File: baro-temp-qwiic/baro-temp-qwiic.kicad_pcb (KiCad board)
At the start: 2 copper layers, 9 x 15 mm, 8 parts, among them J1 Conn_01x04_Male, U1 BMP388, U2 TMP102xxDRL

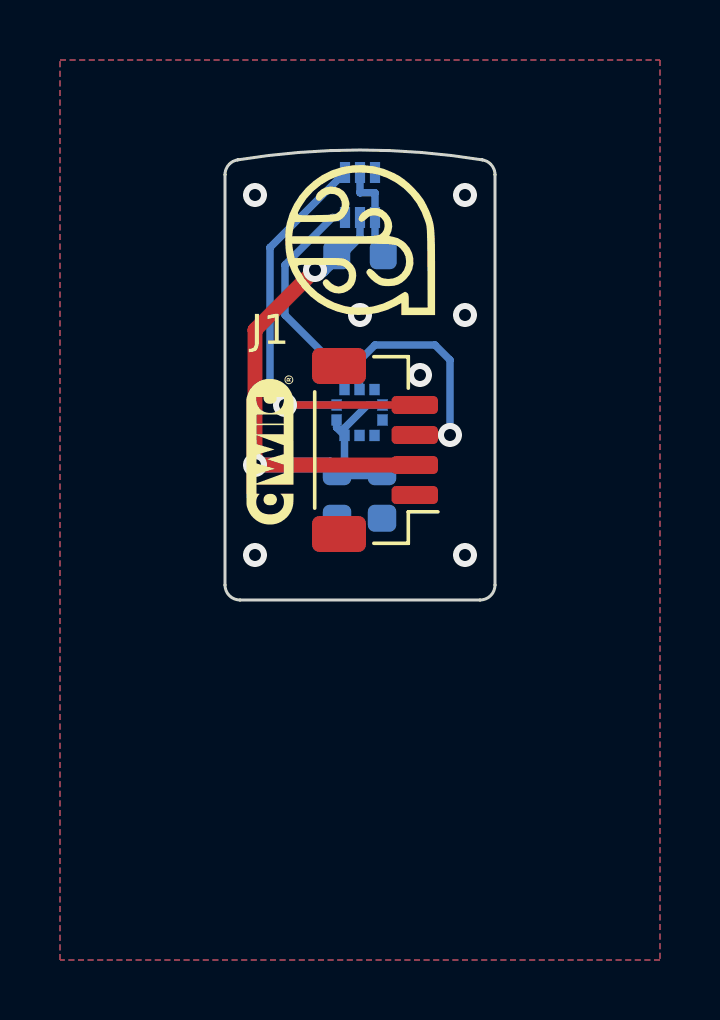
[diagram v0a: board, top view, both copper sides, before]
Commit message: Finished design and made fab outputs.
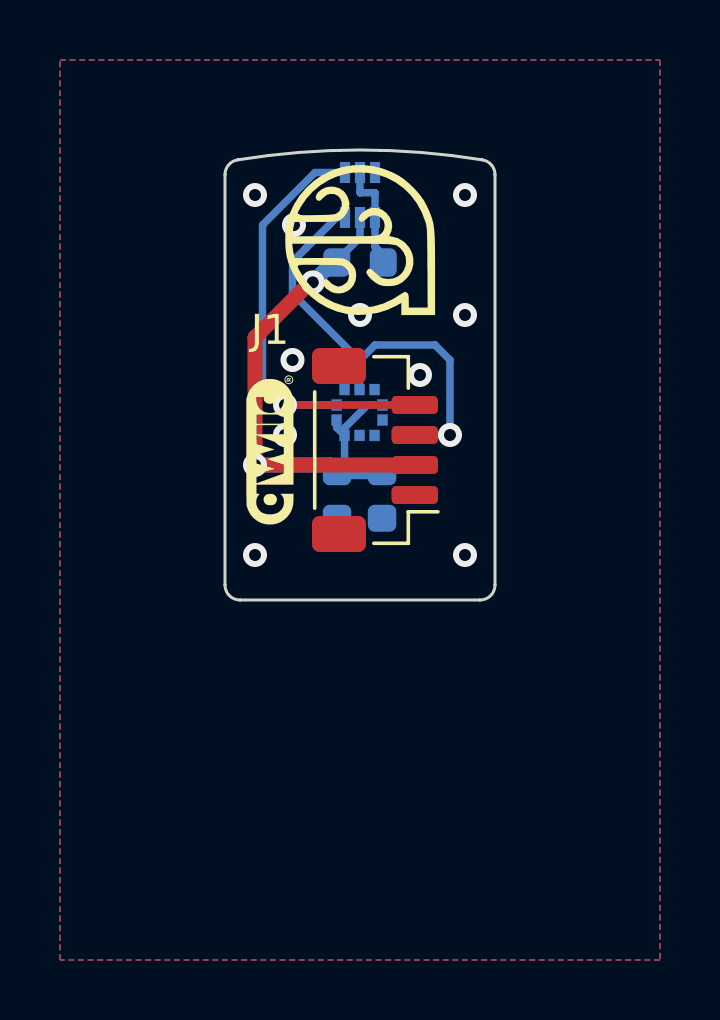
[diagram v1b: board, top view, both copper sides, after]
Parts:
- moved C3 0.25 mm to (0.00, -18.2)
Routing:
- net /SDA: track 15.5 -> 14.7 mm
- net /SCL: track 15.0 -> 15.8 mm
- net GND: vias 7 -> 10
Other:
- board text added: "Airball Temp/Baro 2023-03-14"
- board text added: "Copyright © 2023, The Airball authors"
- board text removed: "Airball Temp/Baro 2023-03-04"
- board text removed: "Copyright (C) 2023, The Airball Authors"
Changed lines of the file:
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@@
       (outputformat 1)
       (mirror false)
-      (drillshape 1)
+      (drillshape 0)
       (scaleselection 1)
       (outputdirectory "")
@@
     (pad "4" smd roundrect (at 1.5 1.325 90) (size 0.6 1.55) (layers "F.Cu" "F.Paste" "F.Mask") (roundrect_rratio 0.25)
       (net 4 "/SCL") (pinfunction "Pin_4") (pintype "passive"))
-    (pad "MP" smd roundrect (at 2.8 -1.2 90) (size 1.2 1.8) (layers "F.Cu" "F.Paste" "F.Mask") (roundrect_rratio 0.208333))
-    (pad "MP" smd roundrect (at -2.8 -1.2 90) (size 1.2 1.8) (layers "F.Cu" "F.Paste" "F.Mask") (roundrect_rratio 0.208333))
+    (pad "MP" smd roundrect (at 2.8 -1.2 90) (size 1.2 1.8) (layers "F.Cu" "F.Paste" "F.Mask") (roundrect_rratio 0.2083333333))
+    (pad "MP" smd roundrect (at -2.8 -1.2 90) (size 1.2 1.8) (layers "F.Cu" "F.Paste" "F.Mask") (roundrect_rratio 0.2083333333))
     (model "/home/ihab/airball-hardware/lib/airball-hardware.pretty/BM04B-SRSS.step"
       (offset (xyz 0 1.25 0))
@@
   )
   (footprint "Capacitor_SMD:C_0603_1608Metric" (layer "B.Cu")
-    (at 0 -18.5)
+    (at 0 -18.25)
     (descr "Capacitor SMD 0603 (1608 Metric), square (rectangular) end terminal, IPC_7351 nominal, (Body size source: IPC-SM-782 page 76, https://www.pcb-3d.com/wordpress/wp-content/uploads/ipc-sm-782a_amendment_1_and_2.pdf), generated with kicad-footprint-generator")
     (tags "capacitor")
@@
   (gr_line (start 4.5 -7.5) (end 4.5 -21.176615) (layer "Edge.Cuts") (width 0.1))
   (gr_arc (start 4.080321 -21.670121) (mid 4.380896 -21.500528) (end 4.5 -21.176615) (layer "Edge.Cuts") (width 0.1))
-  (gr_text "Airball Temp/Baro\n2023-03-04" (at -3 -14.5 90) (layer "B.SilkS")
+  (gr_text "Airball Temp/Baro\n2023-03-14" (at -3 -14.5 90) (layer "B.SilkS")
     (effects (font (size 0.5 0.5) (thickness 0.0625)) (justify mirror))
   )
-  (gr_text "Copyright (C) 2023,\nThe Airball Authors" (at 3 -15 90) (layer "B.SilkS")
+  (gr_text "Copyright © 2023,\nThe Airball authors" (at 3 -15 90) (layer "B.SilkS")
     (effects (font (size 0.5 0.5) (thickness 0.0625)) (justify mirror))
   )
-  (segment (start -3.5 -11.5) (end -3.5 -16) (width 0.5) (layer "F.Cu") (net 1))
-  (segment (start -3.5 -16) (end -1.5 -18) (width 0.5) (layer "F.Cu") (net 1))
+  (segment (start -1.663248 -17.586752) (end -3.5 -15.75) (width 0.5) (layer "F.Cu") (net 1))
+  (segment (start -1.5755 -17.586752) (end -1.663248 -17.586752) (width 0.5) (layer "F.Cu") (net 1))
+  (segment (start -3.5 -15.75) (end -3.5 -11.5) (width 0.5) (layer "F.Cu") (net 1))
   (segment (start 1.825 -11.5) (end -3.5 -11.5) (width 0.5) (layer "F.Cu") (net 1))
   (via (at -3.5 -11.5) (size 0.8) (drill 0.4) (layers "F.Cu" "B.Cu") (net 1))
-  (via (at -1.5 -18) (size 0.8) (drill 0.4) (layers "F.Cu" "B.Cu") (net 1))
+  (via (at -1.5755 -17.586752) (size 0.8) (drill 0.4) (layers "F.Cu" "B.Cu") (net 1))
+  (segment (start -1.5755 -17.586752) (end -0.912252 -18.25) (width 0.5) (layer "B.Cu") (net 1))
   (segment (start -0.780192 -13) (end -0.780192 -12.75) (width 0.25) (layer "B.Cu") (net 1))
   (segment (start -0.765192 -11.275) (end 0.734808 -11.275) (width 0.5) (layer "B.Cu") (net 1))
   (segment (start 0 -19.75) (end 0 -19.08) (width 0.25) (layer "B.Cu") (net 1))
-  (segment (start -1.5 -18) (end -1.275 -18) (width 0.5) (layer "B.Cu") (net 1))
   (segment (start -0.780192 -12.75) (end -0.515192 -12.485) (width 0.25) (layer "B.Cu") (net 1))
   (segment (start 0.25 -13.5) (end 0.749808 -13.5) (width 0.25) (layer "B.Cu") (net 1))
-  (segment (start -1.275 -18) (end -0.775 -18.5) (width 0.5) (layer "B.Cu") (net 1))
-  (segment (start -0.58 -18.5) (end -0.775 -18.5) (width 0.25) (layer "B.Cu") (net 1))
   (segment (start 0 -19.08) (end -0.58 -18.5) (width 0.25) (layer "B.Cu") (net 1))
   (segment (start -0.990192 -11.5) (end -0.765192 -11.275) (width 0.5) (layer "B.Cu") (net 1))
   (segment (start -0.515192 -11.525) (end -0.765192 -11.275) (width 0.25) (layer "B.Cu") (net 1))
+  (segment (start -0.912252 -18.25) (end -0.775 -18.25) (width 0.5) (layer "B.Cu") (net 1))
   (segment (start -0.515192 -12.485) (end -0.515192 -11.525) (width 0.25) (layer "B.Cu") (net 1))
   (segment (start -0.515192 -12.485) (end -0.515192 -12.734808) (width 0.25) (layer "B.Cu") (net 1))
@@
   (segment (start -0.515192 -12.734808) (end 0.25 -13.5) (width 0.25) (layer "B.Cu") (net 1))
   (via (at -3.5 -20.5) (size 0.8) (drill 0.4) (layers "F.Cu" "B.Cu") (free) (net 2))
+  (via (at -2.25 -15) (size 0.8) (drill 0.4) (layers "F.Cu" "B.Cu") (free) (net 2))
   (via (at -3.5 -8.5) (size 0.8) (drill 0.4) (layers "F.Cu" "B.Cu") (free) (net 2))
   (via (at 3.5 -16.5) (size 0.8) (drill 0.4) (layers "F.Cu" "B.Cu") (free) (net 2))
+  (via (at -2.5 -12.5) (size 0.8) (drill 0.4) (layers "F.Cu" "B.Cu") (free) (net 2))
   (via (at 3.5 -8.5) (size 0.8) (drill 0.4) (layers "F.Cu" "B.Cu") (free) (net 2))
   (via (at 2 -14.5) (size 0.8) (drill 0.4) (layers "F.Cu" "B.Cu") (free) (net 2))
   (via (at 3.5 -20.5) (size 0.8) (drill 0.4) (layers "F.Cu" "B.Cu") (free) (net 2))
   (via (at 0 -16.5) (size 0.8) (drill 0.4) (layers "F.Cu" "B.Cu") (free) (net 2))
+  (via (at -2.2 -19.5) (size 0.8) (drill 0.4) (layers "F.Cu" "B.Cu") (free) (net 2))
   (segment (start 0 -21.25) (end 0 -20.58) (width 0.25) (layer "B.Cu") (net 2))
   (segment (start 0.5 -19.75) (end 0.5 -18.775) (width 0.25) (layer "B.Cu") (net 2))
@@
   (segment (start 1.825 -12.5) (end 3 -12.5) (width 0.25) (layer "F.Cu") (net 3))
   (via (at 3 -12.5) (size 0.8) (drill 0.4) (layers "F.Cu" "B.Cu") (net 3))
-  (segment (start -2.5 -18.17) (end -2.5 -16.5) (width 0.25) (layer "B.Cu") (net 3))
-  (segment (start -0.92 -19.75) (end -2.5 -18.17) (width 0.25) (layer "B.Cu") (net 3))
+  (segment (start -0.5 -19.75) (end -0.777817 -19.75) (width 0.25) (layer "B.Cu") (net 3))
   (segment (start -0.015192 -14.984808) (end -0.015192 -14.015) (width 0.25) (layer "B.Cu") (net 3))
-  (segment (start -0.984808 -14.984808) (end -0.015192 -14.984808) (width 0.25) (layer "B.Cu") (net 3))
-  (segment (start -0.5 -19.75) (end -0.92 -19.75) (width 0.25) (layer "B.Cu") (net 3))
+  (segment (start -1.800305 -18.727512) (end -1.800305 -18.725) (width 0.25) (layer "B.Cu") (net 3))
   (segment (start 3 -15) (end 2.5 -15.5) (width 0.25) (layer "B.Cu") (net 3))
   (segment (start 0.5 -15.5) (end -0.015192 -14.984808) (width 0.25) (layer "B.Cu") (net 3))
+  (segment (start -1.800305 -18.725) (end -2.25 -18.275305) (width 0.25) (layer "B.Cu") (net 3))
+  (segment (start -2.25 -18.275305) (end -2.25 -17.219616) (width 0.25) (layer "B.Cu") (net 3))
   (segment (start 3 -12.5) (end 3 -15) (width 0.25) (layer "B.Cu") (net 3))
-  (segment (start -2.5 -16.5) (end -0.984808 -14.984808) (width 0.25) (layer "B.Cu") (net 3))
+  (segment (start -0.777817 -19.75) (end -1.800305 -18.727512) (width 0.25) (layer "B.Cu") (net 3))
   (segment (start 2.5 -15.5) (end 0.5 -15.5) (width 0.25) (layer "B.Cu") (net 3))
+  (segment (start -2.25 -17.219616) (end -0.015192 -14.984808) (width 0.25) (layer "B.Cu") (net 3))
   (segment (start 1.825 -13.5) (end -2.5 -13.5) (width 0.25) (layer "F.Cu") (net 4))
   (via (at -2.5 -13.5) (size 0.8) (drill 0.4) (layers "F.Cu" "B.Cu") (net 4))
+  (segment (start -3.25 -14.25) (end -2.5 -13.5) (width 0.25) (layer "B.Cu") (net 4))
   (segment (start -0.780192 -13.5) (end -2.5 -13.5) (width 0.25) (layer "B.Cu") (net 4))
-  (segment (start -3 -18.75) (end -3 -14) (width 0.25) (layer "B.Cu") (net 4))
-  (segment (start -3 -14) (end -2.5 -13.5) (width 0.25) (layer "B.Cu") (net 4))
-  (segment (start -0.5 -21.25) (end -3 -18.75) (width 0.25) (layer "B.Cu") (net 4))
+  (segment (start -1.5 -21.25) (end -3.25 -19.5) (width 0.25) (layer "B.Cu") (net 4))
+  (segment (start -0.5 -21.25) (end -1.5 -21.25) (width 0.25) (layer "B.Cu") (net 4))
+  (segment (start -3.25 -19.5) (end -3.25 -14.25) (width 0.25) (layer "B.Cu") (net 4))
   (zone (net 2) (net_name "GND") (layers F&B.Cu) (hatch edge 0.508)
     (connect_pads (clearance 0.15))
     (min_thickness 0.15) (filled_areas_thickness no)
-    (fill yes (thermal_gap 0.5) (thermal_bridge_width 0.5))
+    (fill yes (thermal_gap 0.15) (thermal_bridge_width 0.5))
     (polygon
       (pts
